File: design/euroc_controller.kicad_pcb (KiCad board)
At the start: 4 copper layers, 35.1 x 75.7 mm, 88 parts, among them J1 xt30, J2 jst_sh 4, J4 jst_sh 4, J5 jst_sh 4, J6 SMA, J7 Screw_Terminal_01x06, J8 USB_C_Receptacle_USB2.0, J9 jst_sh 4, Q1 MMBT3904, U1 TPSM5601R5, U10 VN7050ASTR, U11 VN7050ASTR, U13 STM32U575CGTx, U2 USBLC6-2SC6, U3 LSM6DSO32, U4 MS5611-01BA, U5 TCAN332, U6 W25Q128JVS, U7 RFM69W, U8 L86, U9 VN7050ASTR, Y1 48MHz

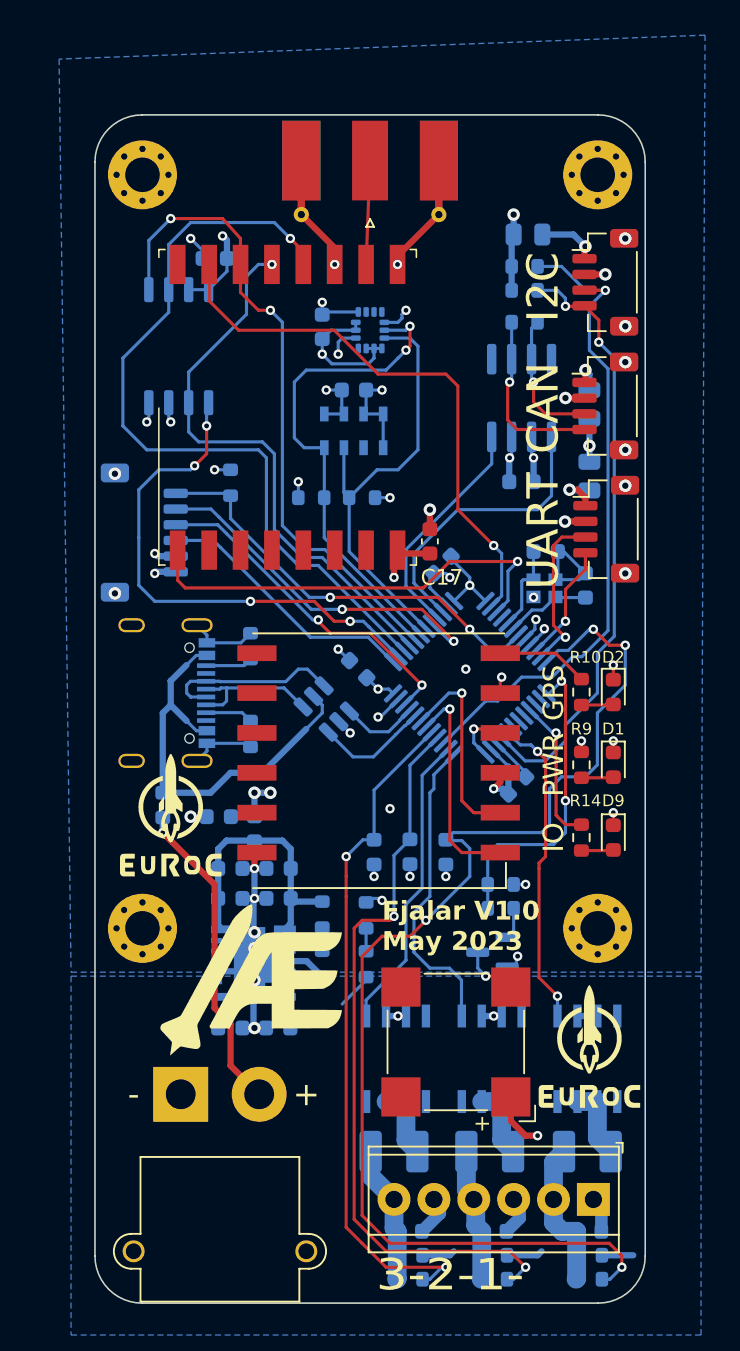
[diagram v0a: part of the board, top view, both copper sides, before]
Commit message: better sma
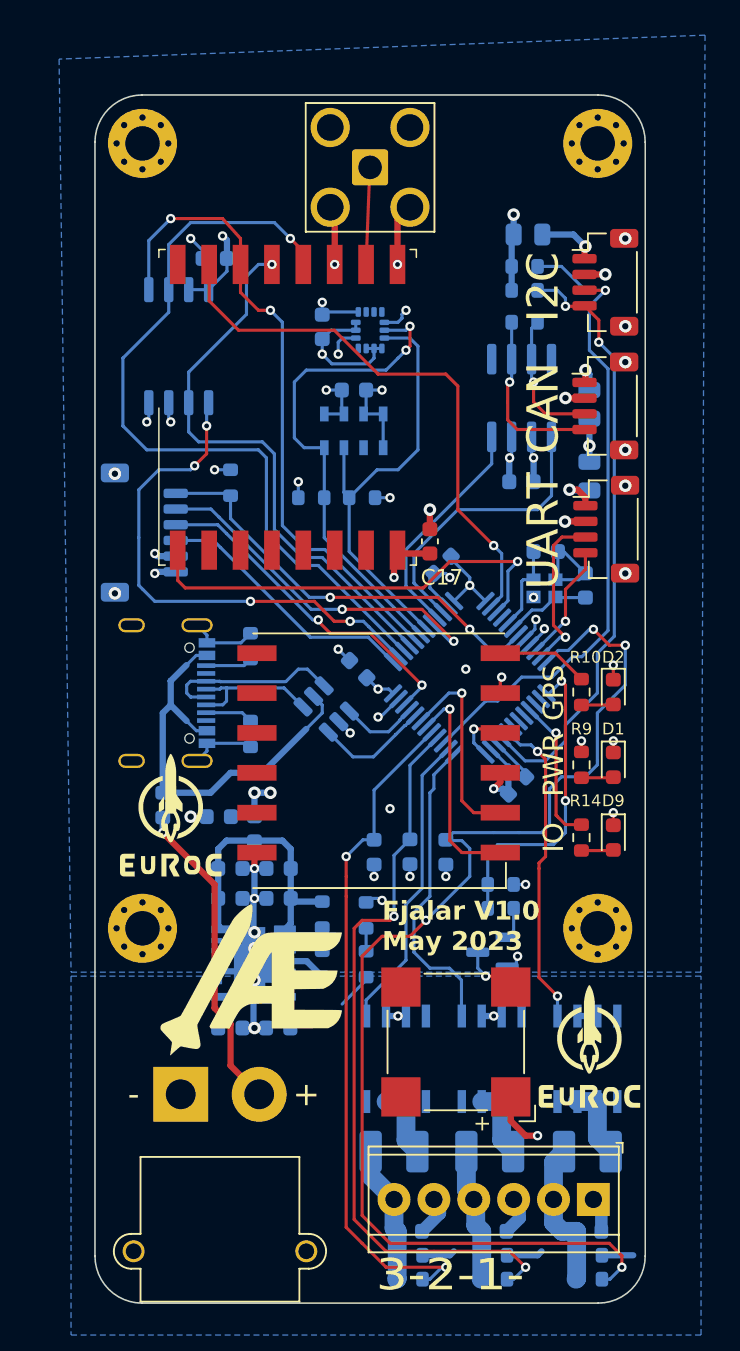
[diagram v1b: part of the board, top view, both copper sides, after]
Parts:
- J6: footprint Connector_Coaxial:SMA_Molex_73251-1153_EdgeMount_Horizontal -> Connector_Coaxial:SMA_Amphenol_901-143_Horizontal
- moved H1 2.00 mm to (167.4, 47.5)
- moved H2 2.00 mm to (196.4, 47.5)
- moved J6 1.29 mm to (181.9, 49.1), turned to 0 degrees
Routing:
- net Earth: track 106.0 -> 105.4 mm
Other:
- board size 35.1 x 75.7 mm -> 35.1 x 77 mm
